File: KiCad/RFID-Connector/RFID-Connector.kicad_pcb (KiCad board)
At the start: 2 copper layers, 90 x 55.5 mm, 10 parts, among them J1 +5V power supply, J2 3V3 RX TX GND, SW1 SW_RESET_TAG_IDs, U1 ESP32-DEVKITC

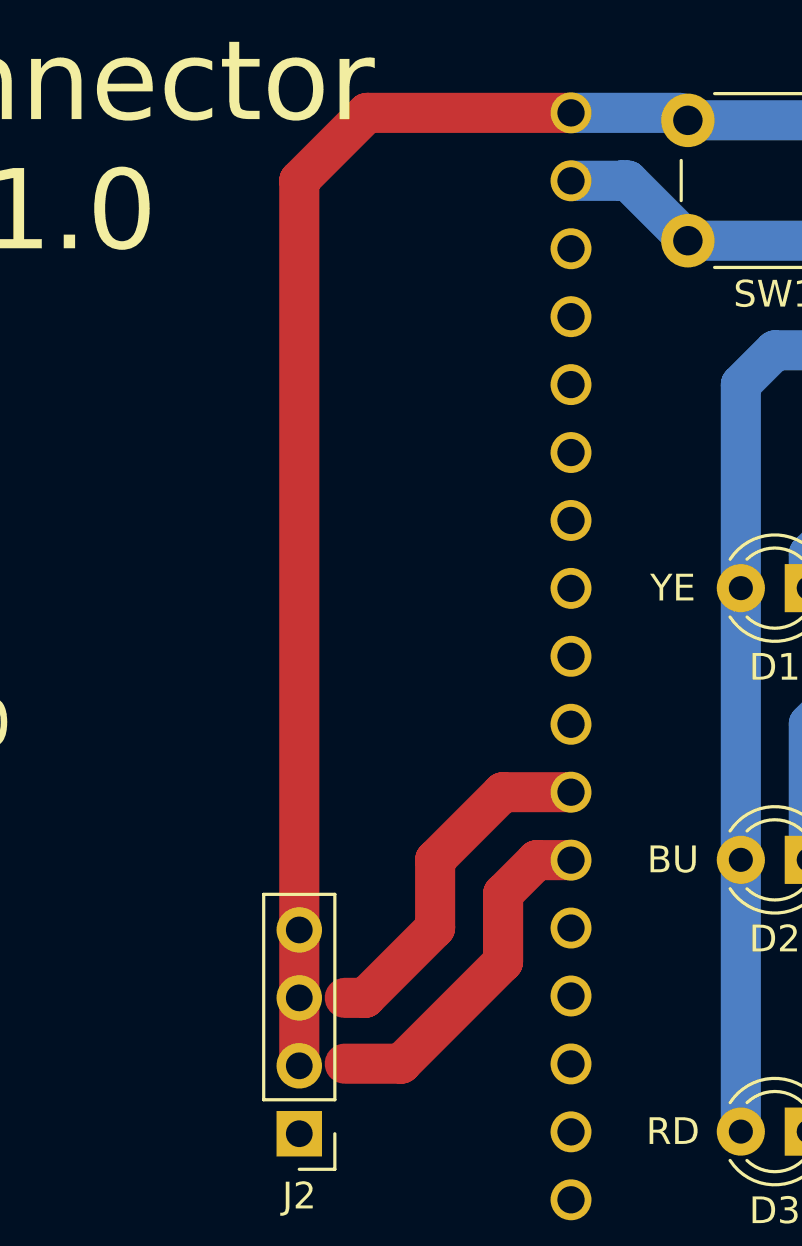
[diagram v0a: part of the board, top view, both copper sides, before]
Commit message: fixed pcb
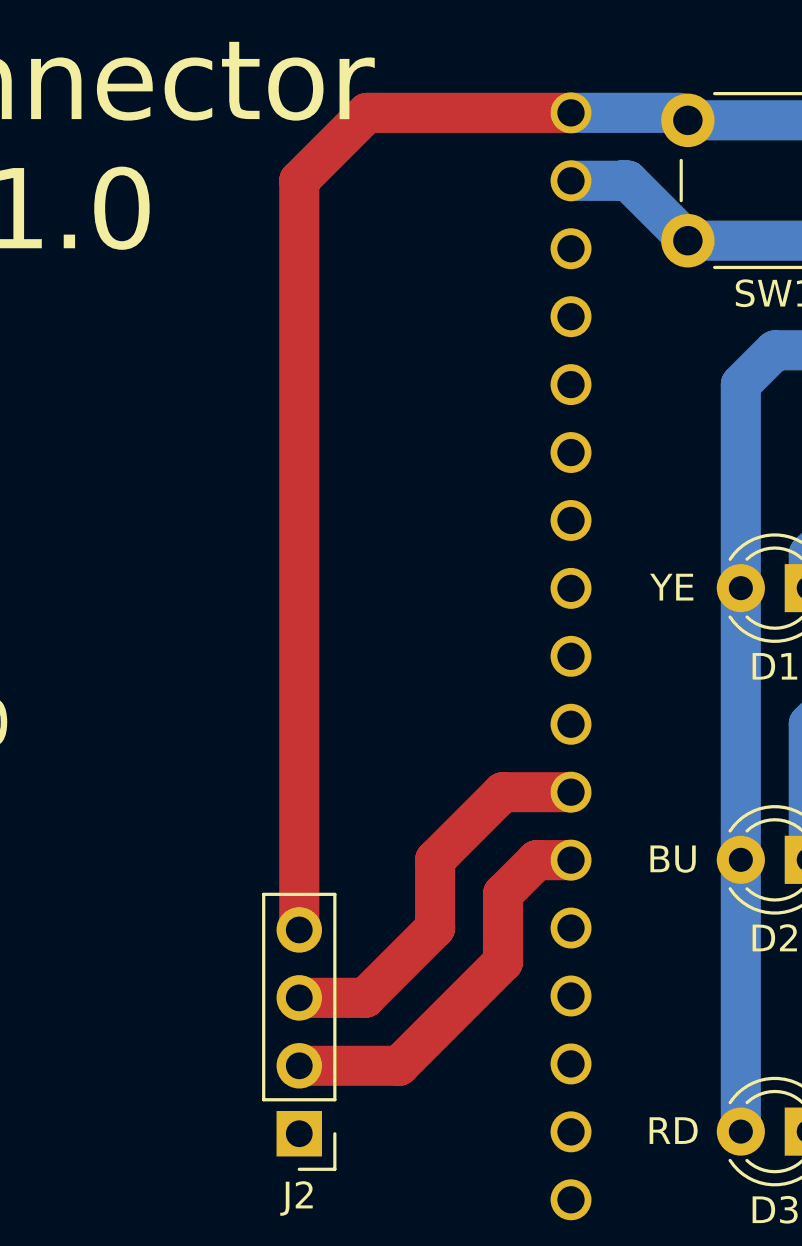
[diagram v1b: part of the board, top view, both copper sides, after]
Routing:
- net Net-(J2-Pad4): track 55.2 -> 50.2 mm
- net Net-(J2-Pad2): track 13.1 -> 14.8 mm
- net Net-(J2-Pad3): track 13.1 -> 14.8 mm
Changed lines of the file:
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@@
   (segment (start 98.345 48.34) (end 94.615 48.34) (width 1.5) (layer "F.Cu") (net 6))
   (segment (start 154.94 73.67) (end 157.47 73.67) (width 1.5) (layer "F.Cu") (net 6))
-  (segment (start 127 59.69) (end 123.19 63.5) (width 1.5) (layer "F.Cu") (net 12))
-  (segment (start 123.19 63.5) (end 121.08 63.5) (width 1.5) (layer "F.Cu") (net 12))
   (segment (start 129.54 55.89) (end 128.26 55.89) (width 1.5) (layer "F.Cu") (net 12))
+  (segment (start 127 57.15) (end 127 59.69) (width 1.5) (layer "F.Cu") (net 12))
+  (segment (start 123.11 63.58) (end 119.38 63.58) (width 1.5) (layer "F.Cu") (net 12))
+  (segment (start 127 59.69) (end 123.11 63.58) (width 1.5) (layer "F.Cu") (net 12))
   (segment (start 128.26 55.89) (end 127 57.15) (width 1.5) (layer "F.Cu") (net 12))
-  (segment (start 127 57.15) (end 127 59.69) (width 1.5) (layer "F.Cu") (net 12))
+  (segment (start 121.84 61.04) (end 119.38 61.04) (width 1.5) (layer "F.Cu") (net 13))
+  (segment (start 124.46 58.42) (end 121.84 61.04) (width 1.5) (layer "F.Cu") (net 13))
   (segment (start 124.46 55.88) (end 124.46 58.42) (width 1.5) (layer "F.Cu") (net 13))
-  (segment (start 121.84 61.04) (end 121.08 61.04) (width 1.5) (layer "F.Cu") (net 13))
   (segment (start 129.54 53.35) (end 126.99 53.35) (width 1.5) (layer "F.Cu") (net 13))
   (segment (start 126.99 53.35) (end 124.46 55.88) (width 1.5) (layer "F.Cu") (net 13))
-  (segment (start 124.46 58.42) (end 121.84 61.04) (width 1.5) (layer "F.Cu") (net 13))
-  (segment (start 119.38 63.5) (end 119.38 30.48) (width 1.5) (layer "F.Cu") (net 14))
   (segment (start 121.91 27.95) (end 129.54 27.95) (width 1.5) (layer "F.Cu") (net 14))
+  (segment (start 119.38 58.5) (end 119.38 30.48) (width 1.5) (layer "F.Cu") (net 14))
   (segment (start 119.38 30.48) (end 121.91 27.95) (width 1.5) (layer "F.Cu") (net 14))
   (segment (start 133.91 28.23) (end 140.41 28.23) (width 1.5) (layer "B.Cu") (net 14))
